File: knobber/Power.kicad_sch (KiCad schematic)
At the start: 3 parts, among them U501 AP2112K-3.3

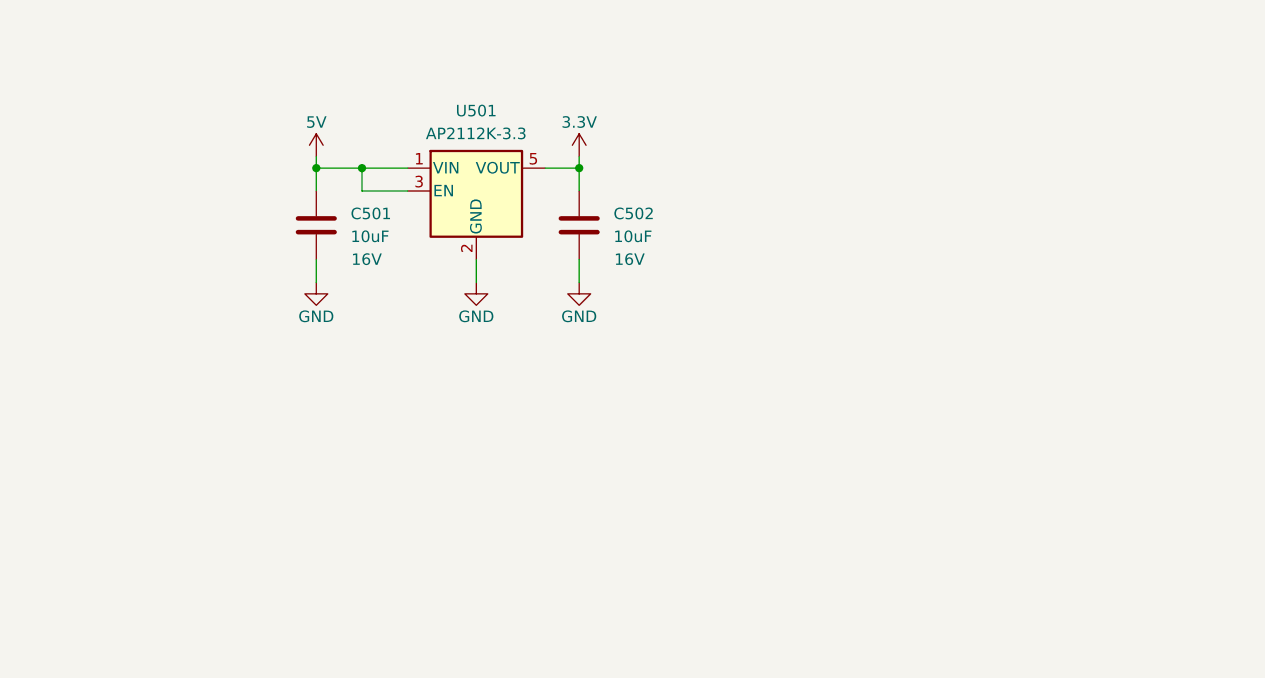
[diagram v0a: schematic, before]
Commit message: Updated schematic & PCB
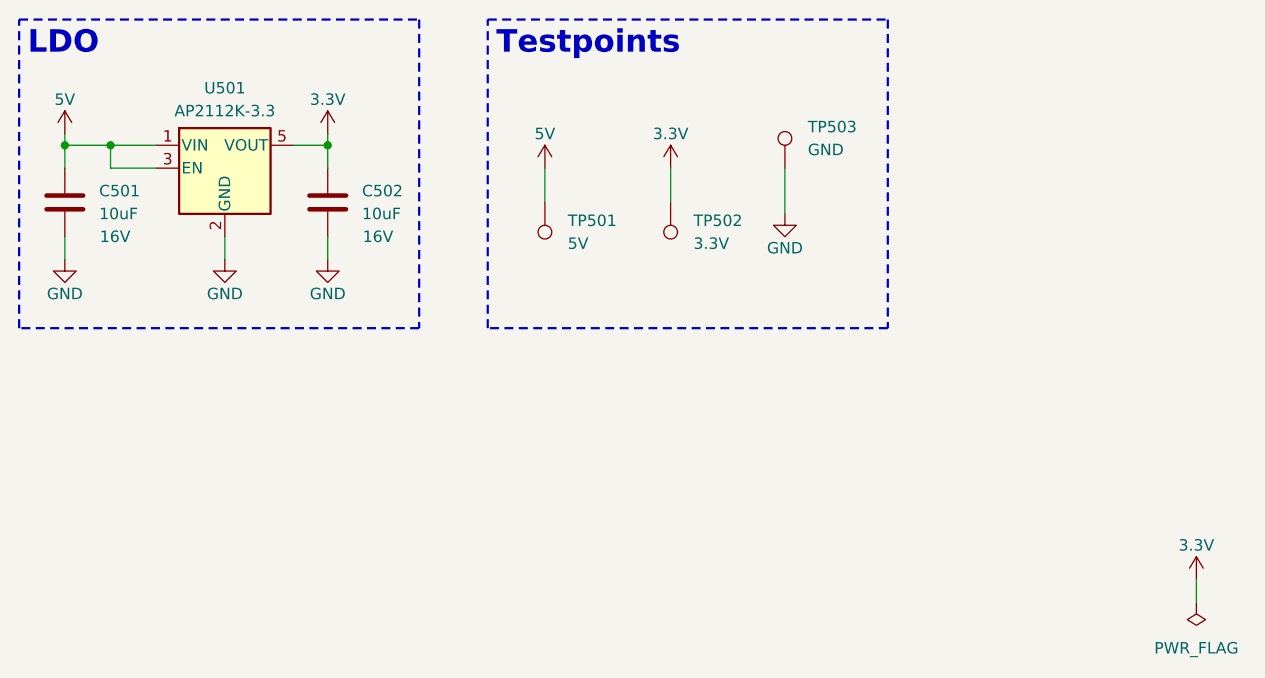
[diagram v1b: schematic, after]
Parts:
- added TP501: 5V, TestPoint:TestPoint_Pad_D1.0mm, symbol Connector:TestPoint
- added TP502: 3.3V, TestPoint:TestPoint_Pad_D1.0mm, symbol Connector:TestPoint
- added TP503: GND, TestPoint:TestPoint_Pad_D1.0mm, symbol Connector:TestPoint
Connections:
- net 3.3V: now also TP502.1
- net 5V: now also TP501.1
- net GND: now also TP503.1
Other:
- moved on the sheet: C501, C502, U501
